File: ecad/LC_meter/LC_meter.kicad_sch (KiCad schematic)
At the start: 29 parts, among them J2 Display Connector, J3 12V Power, U5 LTC1044, U6 LM7805_TO220

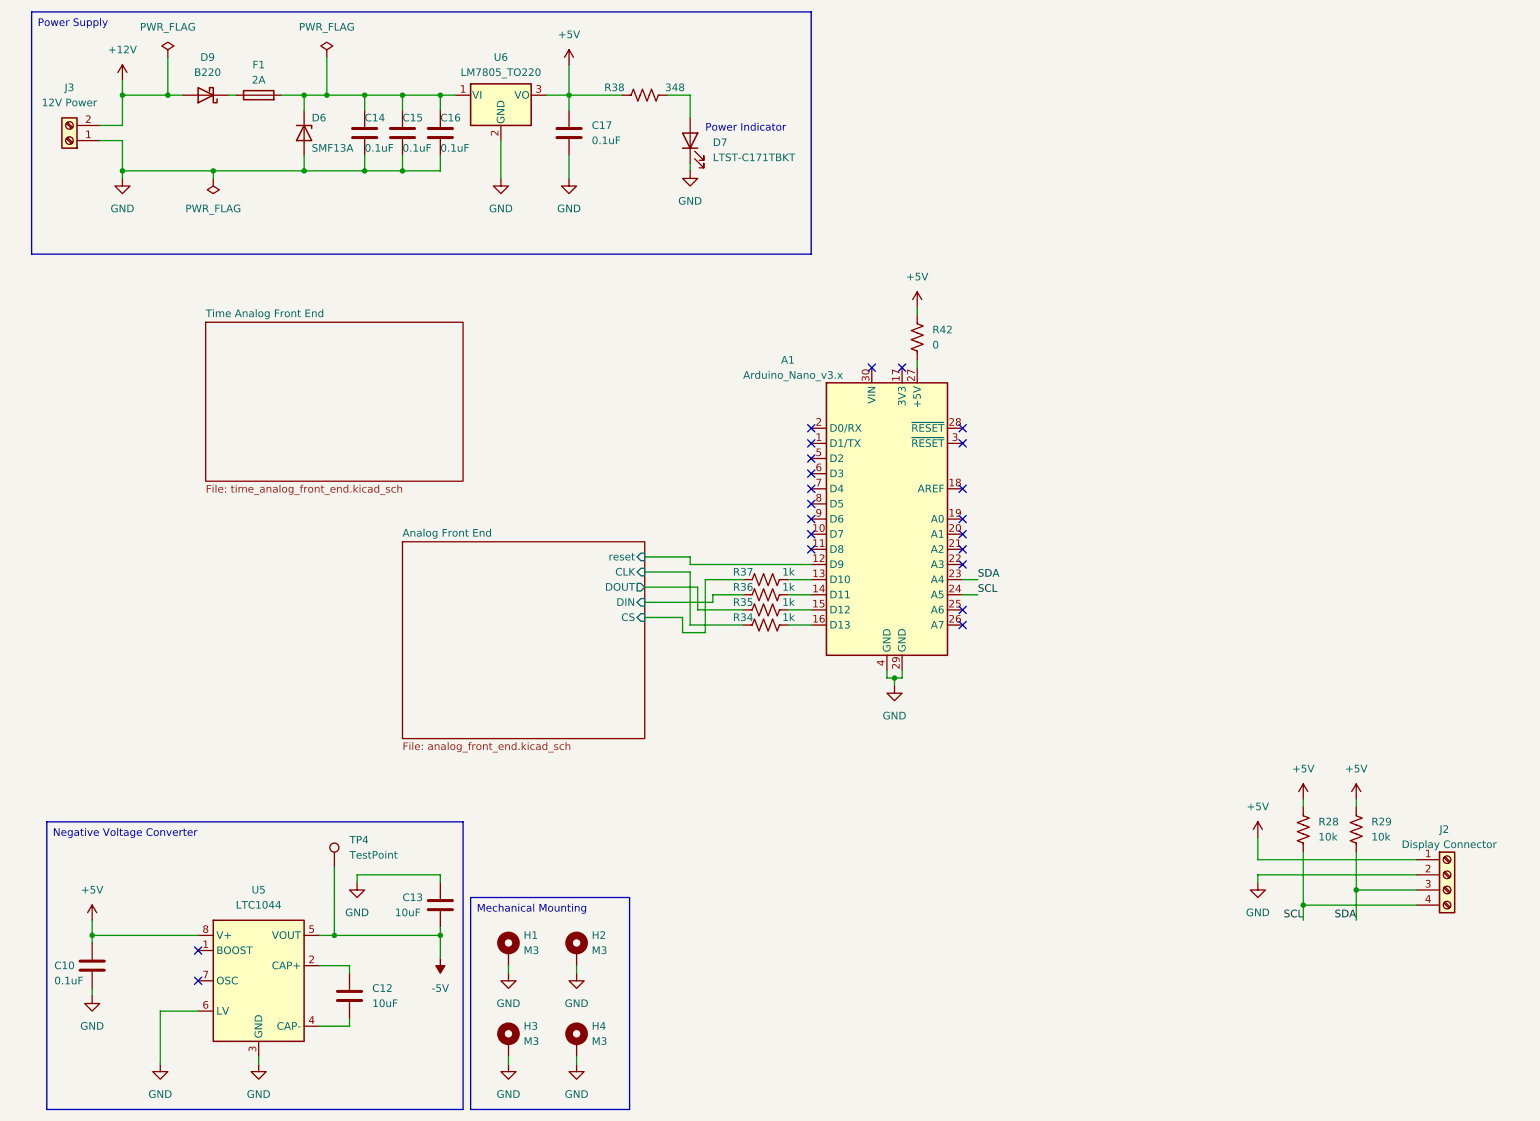
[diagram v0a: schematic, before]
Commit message: time stuff
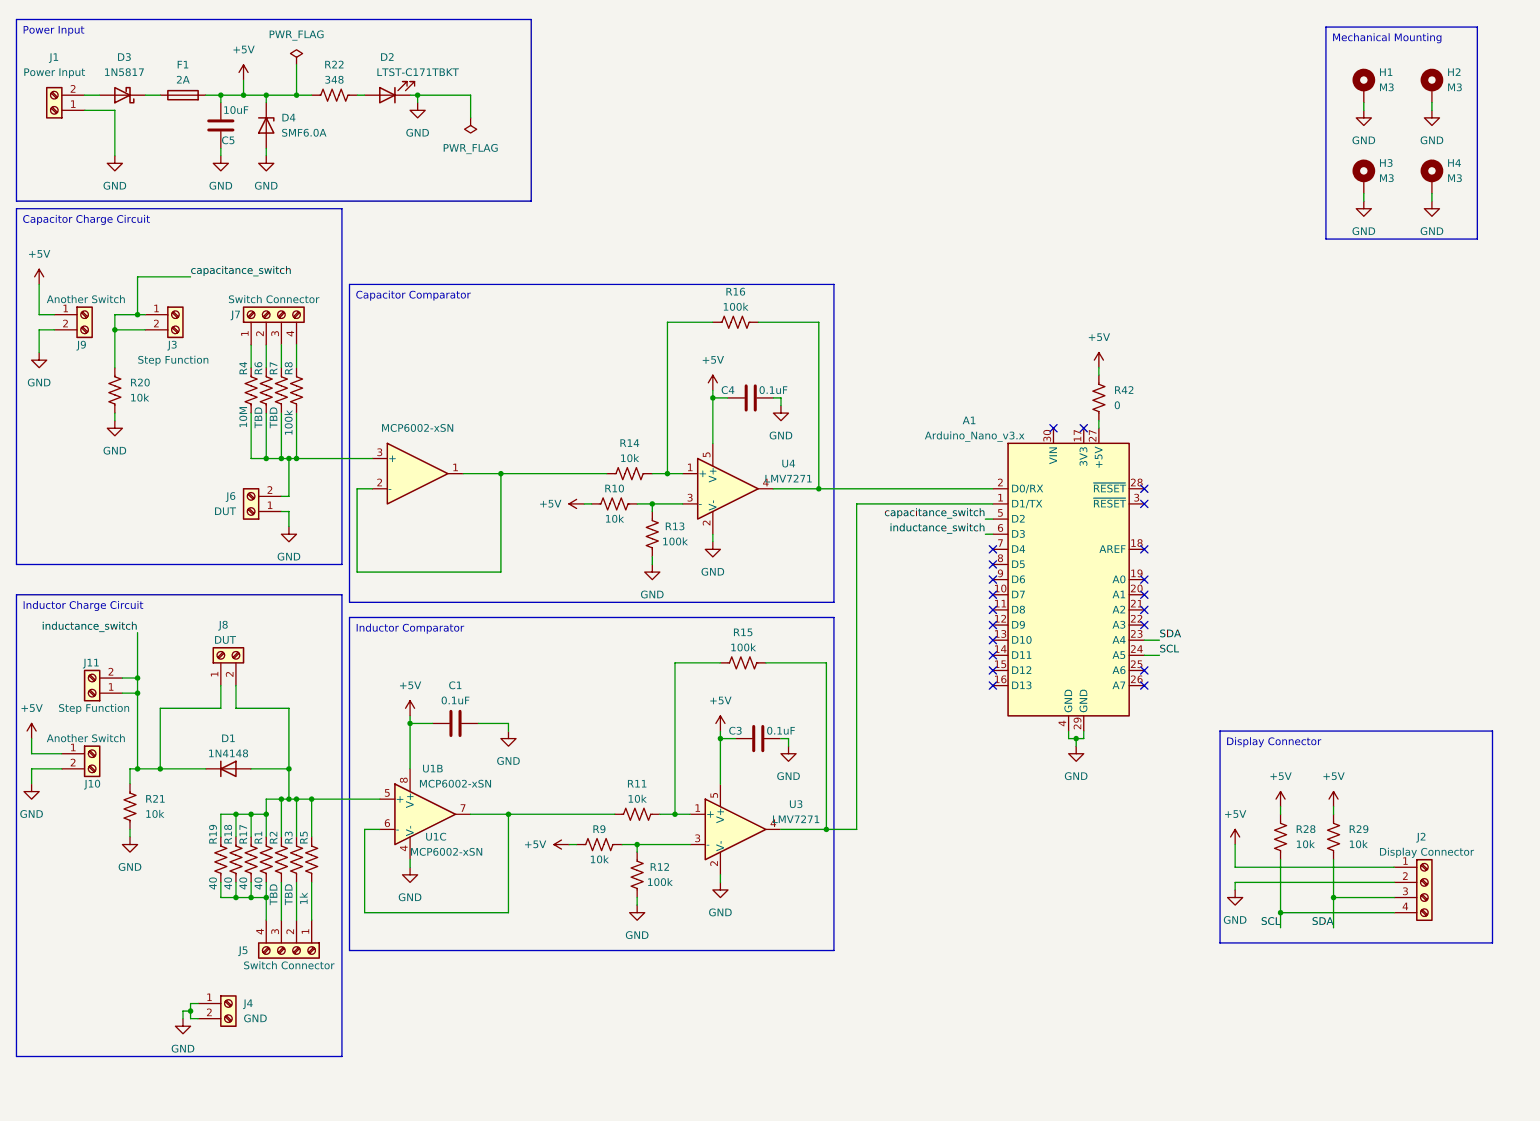
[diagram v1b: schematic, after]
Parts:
- removed C10, C14, C15, C16, C17: 0.1uF, Capacitor_SMD:C_0805_2012Metric, symbol Device:C
- removed C12, C13: 10uF, Capacitor_SMD:C_0805_2012Metric, symbol Device:C
- removed D6: SMF13A, Diode_SMD:D_SMB, symbol Device:D_Zener
- removed D7: LTST-C171TBKT, LED_SMD:LED_0805_2012Metric, symbol Device:LED
- removed D9: B220, Diode_SMD:D_SMB, symbol Diode:B220
- removed R34, R35, R36, R37: 1k, Resistor_SMD:R_0805_2012Metric, symbol Device:R_US
- removed R38: 348, Resistor_SMD:R_0805_2012Metric, symbol Device:R_US
- removed TP4: TestPoint, symbol Connector:TestPoint
- removed U5: LTC1044, symbol Regulator_SwitchedCapacitor:LTC1044
- removed U6: LM7805_TO220, Package_TO_SOT_THT:TO-220-3_Vertical, symbol Regulator_Linear:LM7805_TO220
- added C1, C3, C4: 0.1uF, Capacitor_SMD:C_0805_2012Metric, symbol Device:C
- added C5: 10uF, Capacitor_SMD:C_0805_2012Metric, symbol Device:C
- added D1: 1N4148, Diode_THT:D_DO-35_SOD27_P7.62mm_Horizontal, symbol Diode:1N4148
- added D2: LTST-C171TBKT, LED_SMD:LED_0805_2012Metric, symbol Device:LED
- added D3: 1N5817, Diode_THT:D_DO-41_SOD81_P10.16mm_Horizontal, symbol Diode:1N5817
- added D4: SMF6.0A, Diode_SMD:D_SOD-123, symbol Device:D_Zener
- added J1: Power Input, TerminalBlock_Phoenix:TerminalBlock_Phoenix_MPT-0,5-2-2.54_1x02_P2.54mm_Horizontal, symbol Connector:Screw_Terminal_01x02
- added J10, J9: Another Switch, TerminalBlock_Phoenix:TerminalBlock_Phoenix_MPT-0,5-2-2.54_1x02_P2.54mm_Horizontal, symbol Connector:Screw_Terminal_01x02
- added J11: Step Function, TerminalBlock_Phoenix:TerminalBlock_Phoenix_MPT-0,5-2-2.54_1x02_P2.54mm_Horizontal, symbol Connector:Screw_Terminal_01x02
- added J4: GND, TerminalBlock_Phoenix:TerminalBlock_Phoenix_MPT-0,5-2-2.54_1x02_P2.54mm_Horizontal, symbol Connector:Screw_Terminal_01x02
- added J5, J7: Switch Connector, TerminalBlock_Phoenix:TerminalBlock_Phoenix_MPT-0,5-4-2.54_1x04_P2.54mm_Horizontal, symbol Connector:Screw_Terminal_01x04
- added J6, J8: DUT, TerminalBlock_Phoenix:TerminalBlock_Phoenix_MPT-0,5-2-2.54_1x02_P2.54mm_Horizontal, symbol Connector:Screw_Terminal_01x02
- added R1, R17, R18, R19: 40, Resistor_SMD:R_0805_2012Metric, symbol Device:R_US
- added R10, R11, R14, R20, R21, R9: 10k, Resistor_SMD:R_0805_2012Metric, symbol Device:R_US
- added R12, R13, R15, R16, R8: 100k, Resistor_SMD:R_0805_2012Metric, symbol Device:R_US
- added R2, R3, R6, R7: TBD, Resistor_SMD:R_0805_2012Metric, symbol Device:R_US
- added R22: 348, Resistor_SMD:R_0805_2012Metric, symbol Device:R_US
- added R4: 10M, Resistor_SMD:R_0805_2012Metric, symbol Device:R_US
- added R5: 1k, Resistor_SMD:R_0805_2012Metric, symbol Device:R_US
- added U1: MCP6002-xSN, Package_SO:SOIC-8_3.9x4.9mm_P1.27mm, symbol Amplifier_Operational:MCP6002-xSN
- added U3, U4: LMV7271, Package_TO_SOT_SMD:SOT-23-5, symbol Comparator:LMV7271
- J2: footprint (none) -> TerminalBlock_Phoenix:TerminalBlock_Phoenix_MPT-0,5-4-2.54_1x04_P2.54mm_Horizontal
- J3: value 12V Power -> Step Function; footprint (none) -> TerminalBlock_Phoenix:TerminalBlock_Phoenix_MPT-0,5-2-2.54_1x02_P2.54mm_Horizontal
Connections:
- net +12V is gone; now on net capacitance_switch: J3.2 (Pin_2)
- net +5V: now also F1.2, C1.1, C3.1, C4.1, C5.2, D4.1 (K), J10.1 (Pin_1), J9.1 (Pin_1), R10.1, R22.1, R9.1, U1.8 (V+), U3.5 (V+), U4.5 (V+)
- net GND: now also C1.2, C3.2, C4.2, C5.1, D2.1 (K), D4.2 (A), J1.1 (Pin_1), J10.2 (Pin_2), J4.1 (Pin_1), J4.2 (Pin_2), J6.1 (Pin_1), J9.2 (Pin_2), R12.1, R13.1, R20.2, R21.2, U1.4 (V-), U3.2 (V-), U4.2 (V-); no longer J3.1 (Pin_1)
- net at F1.1: now also D3.1 (K)
- net at A1.1 (D1/TX): now also R15.2, U3.4
- net at A1.2 (D0/RX): now also R16.2, U4.4
- net capacitance_switch: now reaches A1.5 (D2)
- net capacitance_switch: now also J3.1 (Pin_1), R20.1
- net inductance_switch: now reaches A1.6 (D3)
- net inductance_switch: now also D1.1 (K), J11.1 (Pin_1), J11.2 (Pin_2), J8.1 (Pin_1), R21.1
- net Analog Front End/reset: no longer names the net of A1.12 (D9)
- new net: J5.1 (Pin_1), R5.2
- new net: J5.2 (Pin_2), R3.2
- new net: J5.3 (Pin_3), R2.2
- new net: J5.4 (Pin_4), R1.2, R17.2, R18.2, R19.2
- new net: R10.2, R13.2, U4.3 (-)
- new net: R11.1, U1.6 (-), U1.7
- new net: R11.2, R15.1, U3.1 (+)
- new net: D1.2 (A), J8.2 (Pin_2), R1.1, R17.1, R18.1, R19.1, R2.1, R3.1, R5.1, U1.5 (+)
- new net: R12.2, R9.2, U3.3 (-)
- new net: D2.2 (A), R22.2
- new net: D3.2 (A), J1.2 (Pin_2)
- new net: R14.1, U1.1, U1.2 (-)
- new net: J6.2 (Pin_2), R4.2, R6.2, R7.2, R8.2, U1.3 (+)
- new net: J7.1 (Pin_1), R4.1
- new net: J7.2 (Pin_2), R6.1
- new net: J7.3 (Pin_3), R7.1
- new net: J7.4 (Pin_4), R8.1
- new net: R14.2, R16.1, U4.1 (+)
- no-connect marks 22 -> 21
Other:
- removed sheet Analog Front End
- removed sheet Time Analog Front End
- note removed: "Power Indicator"
- moved on the sheet: A1, H1, H2, H3, H4, J2, R28, R29, R42
